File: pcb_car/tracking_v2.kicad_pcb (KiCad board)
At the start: 2 copper layers, 75 x 64 mm, 28 parts, among them J1 Conn_01x02, J2 Conn_01x02, J3 Conn_01x02, J4 Conn_01x02, J5 Conn_01x16_Female, J6 Conn_01x02, J7 Conn_01x20_Female, J8 Conn_01x03, J9 Conn_01x03, SW1 SW_Push, U1 L293D, U2 L293D, U3 GY-521

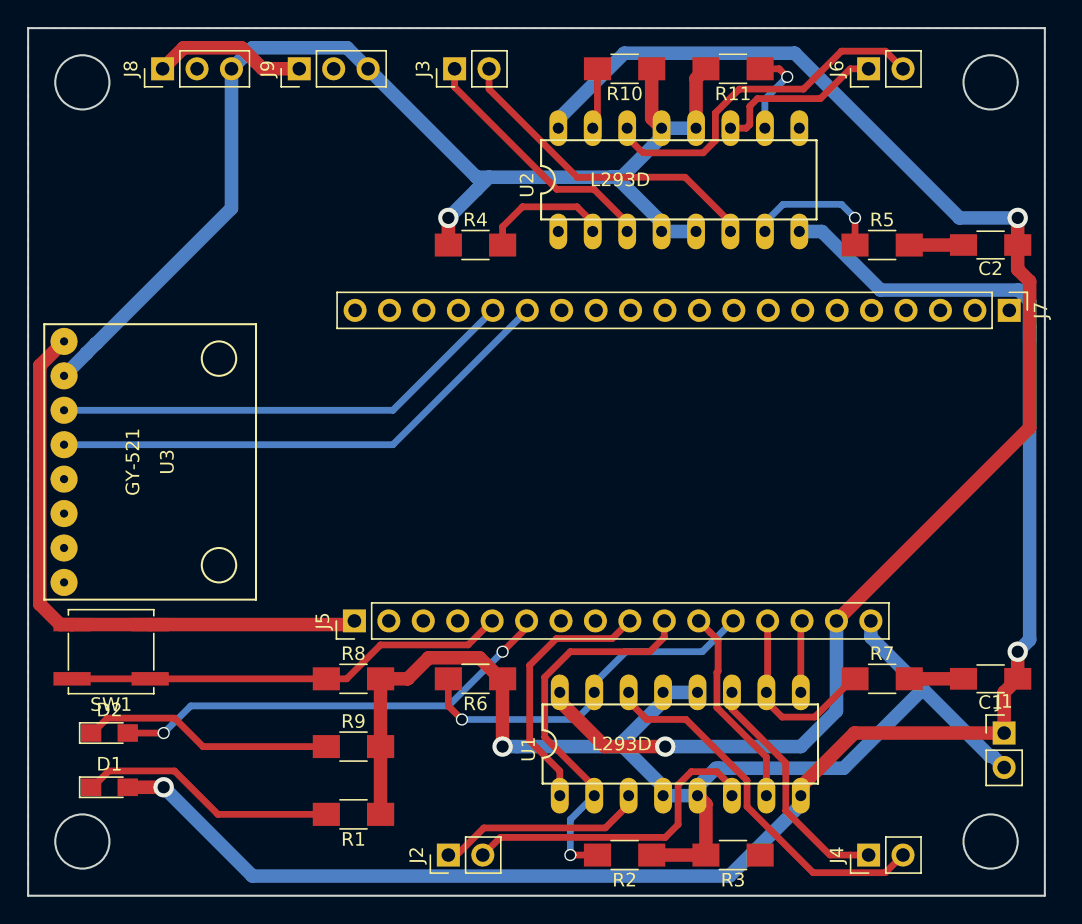
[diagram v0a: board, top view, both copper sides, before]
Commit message: Finished second iteration of PCB
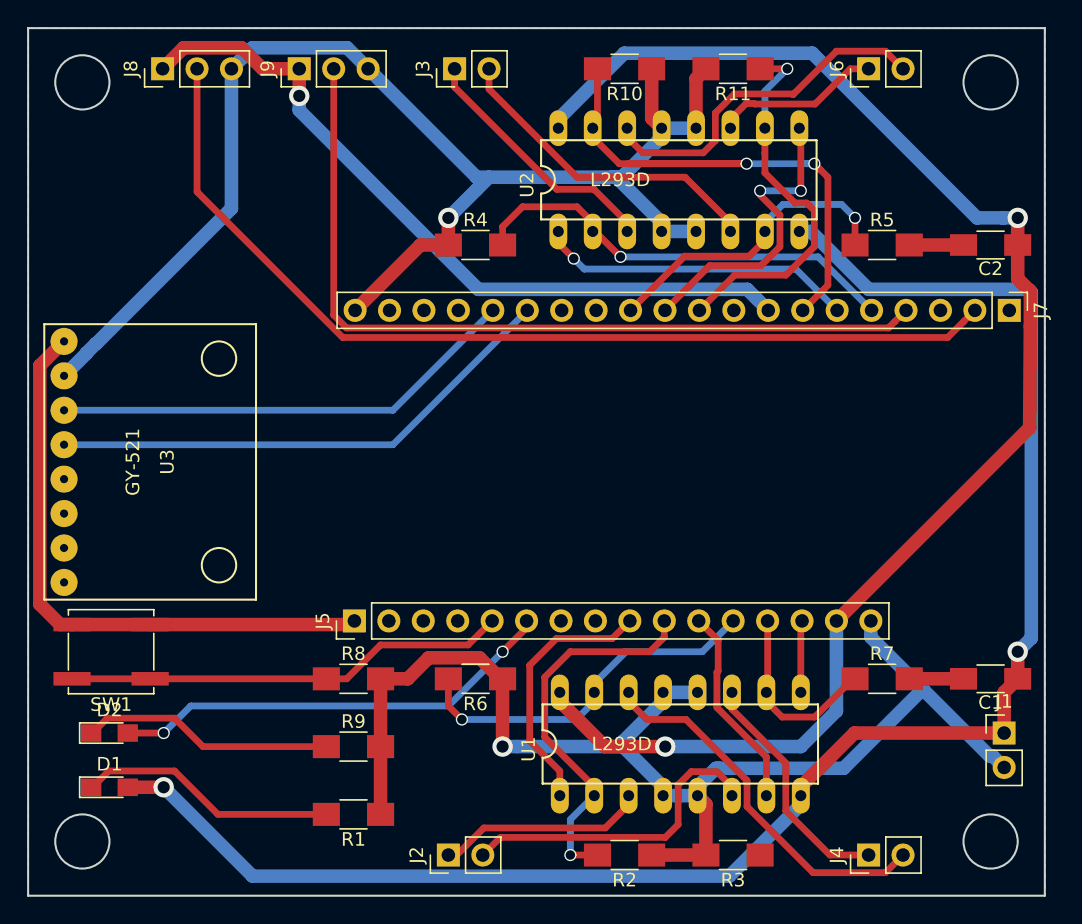
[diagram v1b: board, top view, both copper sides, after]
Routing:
- net DATA2: track 0.00 -> 71.7 mm
- net DATA1: track 0.00 -> 61.3 mm
- net 3V3: track 11.4 -> 55.1 mm, vias 0 -> 1
- net IN4_B: track 5.19 -> 43.7 mm, vias 0 -> 2
- net EN1_B: track 0.00 -> 23.5 mm, vias 0 -> 1
- net IN1_B: track 9.75 -> 32.7 mm, vias 0 -> 1
- net EN2_B: track 0.66 -> 23.5 mm, vias 0 -> 2
- net IN3_B: track 7.37 -> 28.5 mm
- net IN2_B: track 10.3 -> 23.0 mm
- net GND: track 195.7 -> 204.5 mm
- net BATT: track 125.4 -> 124.8 mm
